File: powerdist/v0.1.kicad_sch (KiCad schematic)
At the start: 11 parts

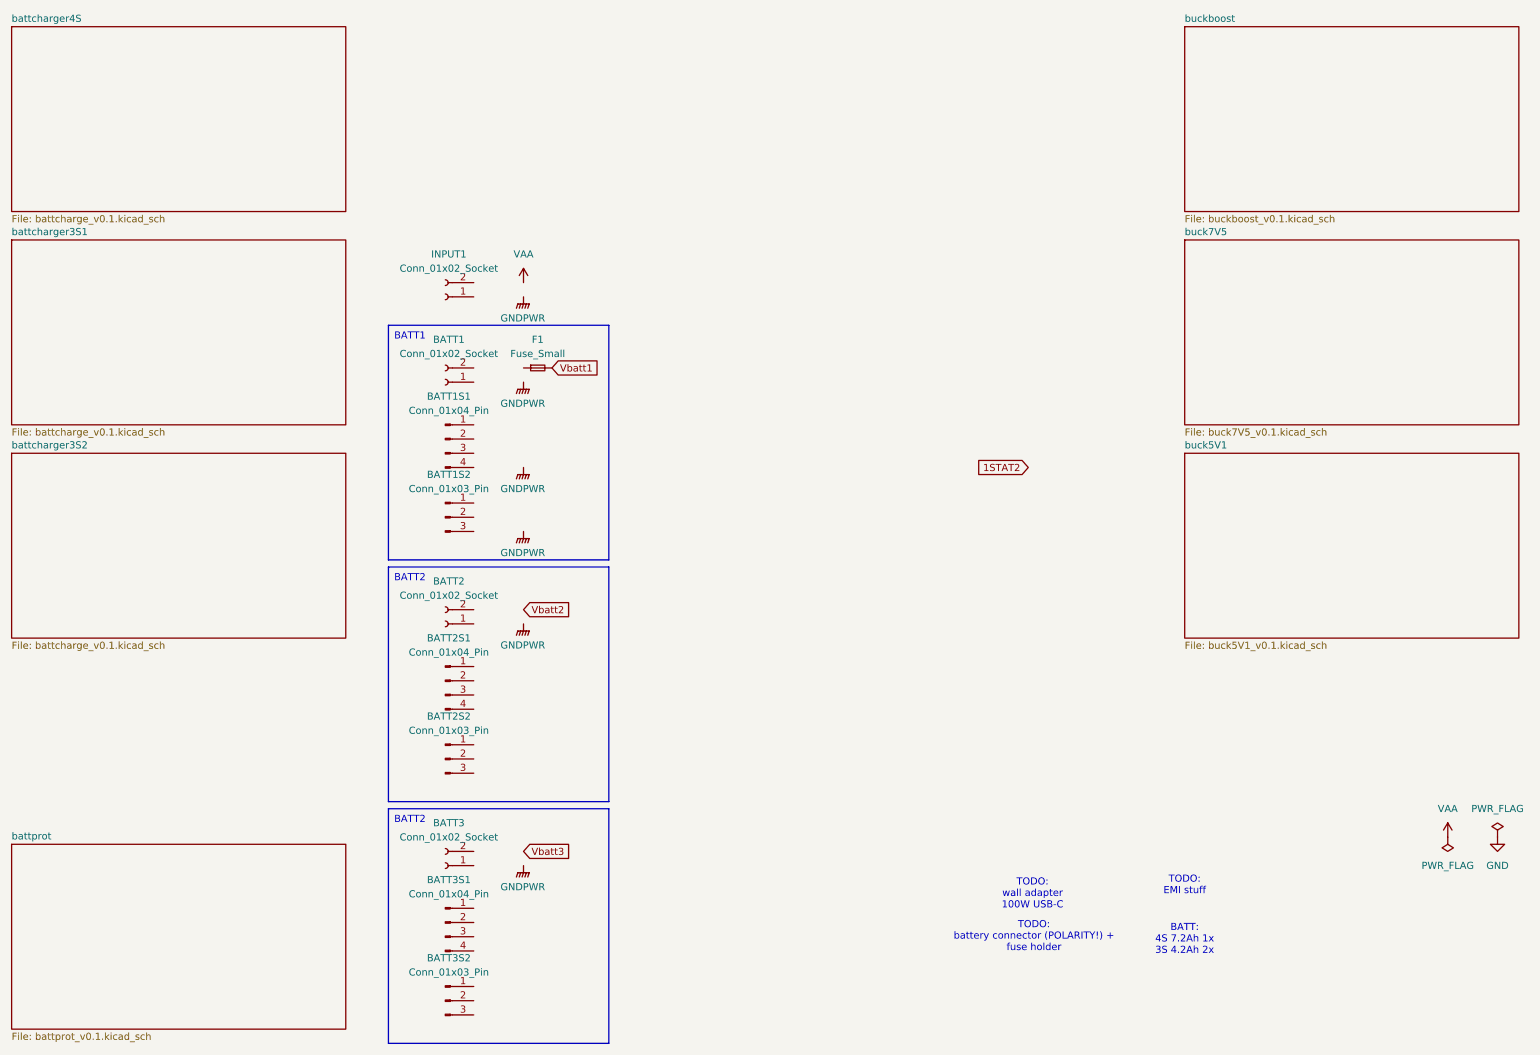
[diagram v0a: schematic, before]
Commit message: lab 02/10
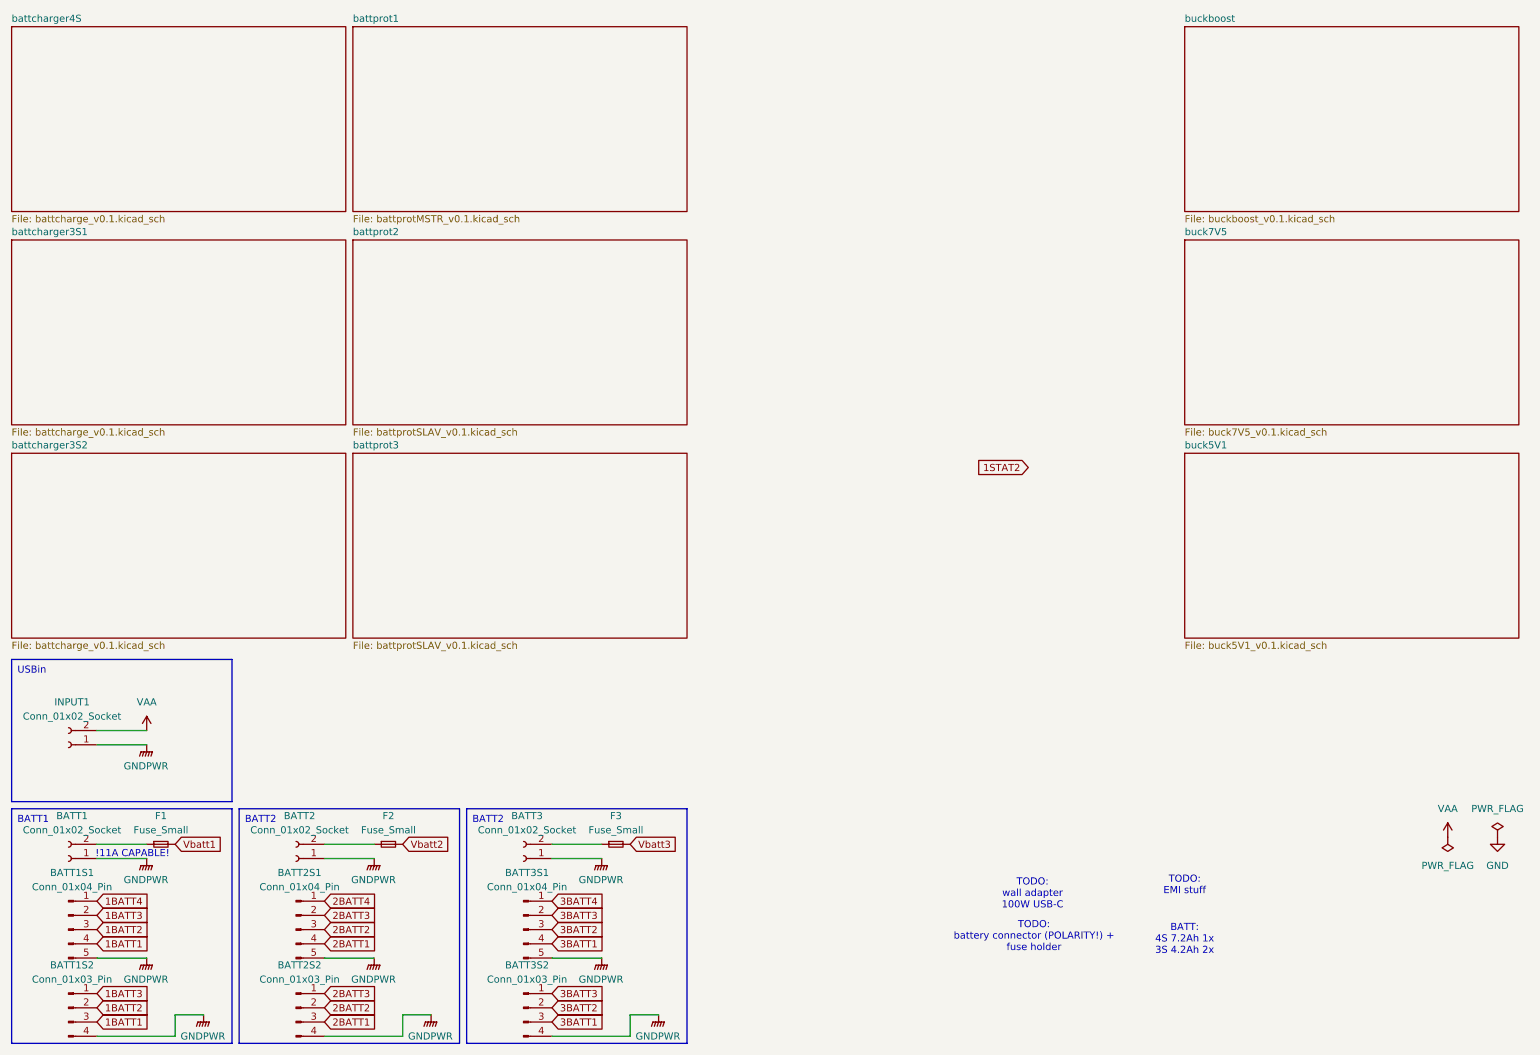
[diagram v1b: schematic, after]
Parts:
- added F2, F3: Fuse_Small, symbol Device:Fuse_Small
- BATT1S1, BATT2S1, BATT3S1: symbol Connector:Conn_01x04_Pin -> Connector:Conn_01x05_Pin
- BATT1S2, BATT2S2, BATT3S2: symbol Connector:Conn_01x03_Pin -> Connector:Conn_01x04_Pin
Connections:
- net GNDPWR: now also BATT1.1 (Pin_1), BATT1S1.5 (Pin_5), BATT1S2.4 (Pin_4), BATT2.1 (Pin_1), BATT2S1.5 (Pin_5), BATT2S2.4 (Pin_4), BATT3.1 (Pin_1), BATT3S1.5 (Pin_5), BATT3S2.4 (Pin_4), INPUT1.1 (Pin_1)
- net VAA: now also INPUT1.2 (Pin_2)
- net Vbatt2: now also F2.2
- net Vbatt3: now also F3.2
- net at BATT1.2 (Pin_2): now also F1.1
- net at BATT2.2 (Pin_2): now also F2.1
- net 3BATT3: now reaches BATT3S2.1 (Pin_1)
- net 3BATT3: now also BATT3S1.2 (Pin_2)
- net 3BATT2: now reaches BATT3S2.2 (Pin_2)
- net 3BATT2: now also BATT3S1.3 (Pin_3)
- net 3BATT1: now reaches BATT3S2.3 (Pin_3)
- net 3BATT1: now also BATT3S1.4 (Pin_4)
- net 3BATT4: now reaches BATT3S1.1 (Pin_1)
- net 2BATT4: now reaches BATT2S1.1 (Pin_1)
- net 2BATT3: now reaches BATT2S1.2 (Pin_2)
- net 2BATT3: now also BATT2S2.1 (Pin_1)
- net 2BATT2: now reaches BATT2S1.3 (Pin_3)
- net 2BATT2: now also BATT2S2.2 (Pin_2)
- net 2BATT1: now reaches BATT2S1.4 (Pin_4)
- net 2BATT1: now also BATT2S2.3 (Pin_3)
- net at BATT3.2 (Pin_2): now also F3.1
- net 1BATT3: now reaches BATT1S2.1 (Pin_1)
- net 1BATT3: now also BATT1S1.2 (Pin_2)
- net 1BATT2: now reaches BATT1S2.2 (Pin_2)
- net 1BATT2: now also BATT1S1.3 (Pin_3)
- net 1BATT1: now reaches BATT1S2.3 (Pin_3)
- net 1BATT1: now also BATT1S1.4 (Pin_4)
- net 1BATT4: now reaches BATT1S1.1 (Pin_1)
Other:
- sheet battprot renamed battprot1
- added sheet battprot2 (battprotSLAV_v0.1.kicad_sch)
- added sheet battprot3 (battprotSLAV_v0.1.kicad_sch)
- sheet battprot1: file battprot_v0.1.kicad_sch -> battprotMSTR_v0.1.kicad_sch
- note added: "!11A CAPABLE!"
- moved on the sheet: BATT1, BATT2, BATT3, F1, INPUT1
